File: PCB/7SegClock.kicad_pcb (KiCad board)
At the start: 2 copper layers, 177.8 x 76.2 mm, 144 parts, among them CON1 USB_Micro_Vertical, Q1 NPN, Q10 DMN2041LSD-13, Q11 DMN2041LSD-13, Q12 DMN2041LSD-13, Q13 DMN2041LSD-13, Q14 DMN2041LSD-13, Q15 DMN2041LSD-13, Q16 DMN2041LSD-13, Q17 DMN2041LSD-13, Q18 DMN2041LSD-13, Q19 DMN2041LSD-13, Q2 DMN2041LSD-13, Q20 DMN2041LSD-13, Q21 DMN2041LSD-13, Q22 DMN2041LSD-13, Q23 DMN2041LSD-13, Q24 DMN2041LSD-13, Q25 DMN2041LSD-13, Q26 DMN2041LSD-13, Q27 DMN2041LSD-13, Q28 DMN2041LSD-13, Q29 DMN2041LSD-13, Q3 DMN2041LSD-13, Q30 DMN2041LSD-13, Q31 DMN2041LSD-13, Q32 DMN2041LSD-13, Q4 DMN2041LSD-13, Q5 DMN2041LSD-13, Q6 DMN2041LSD-13, Q7 DMN2041LSD-13, Q8 DMN2041LSD-13, Q9 DMN2041LSD-13, U1 TPS62172DSGT, U2 P8X32A, U3 FT232RL, U4 24LC256, U5 DS3231, U6 LCMX02-640UHC-4TG144C, U7 Electric_Imp, X1 5mhz CRYSTAL

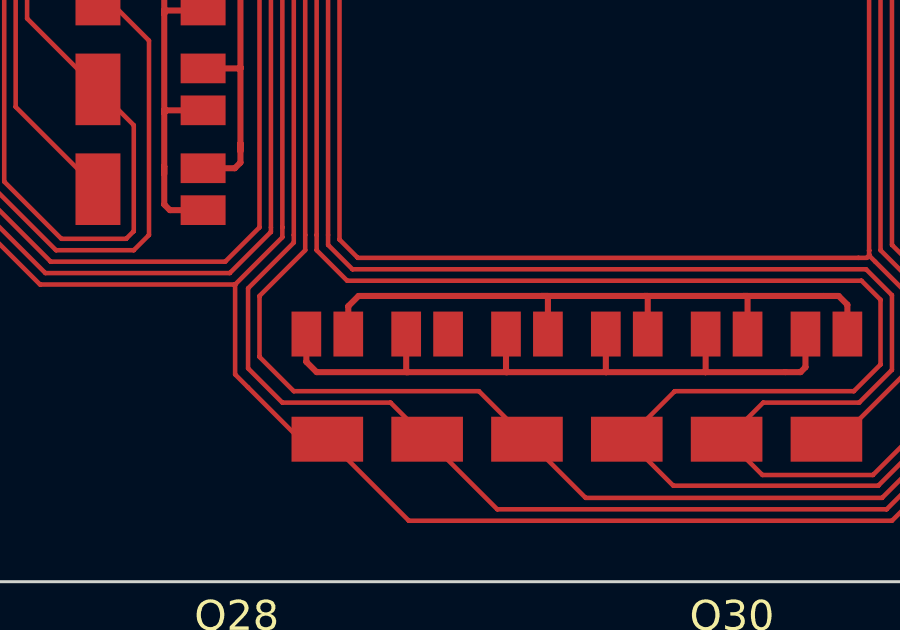
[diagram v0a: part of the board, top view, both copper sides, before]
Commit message: PCB work.
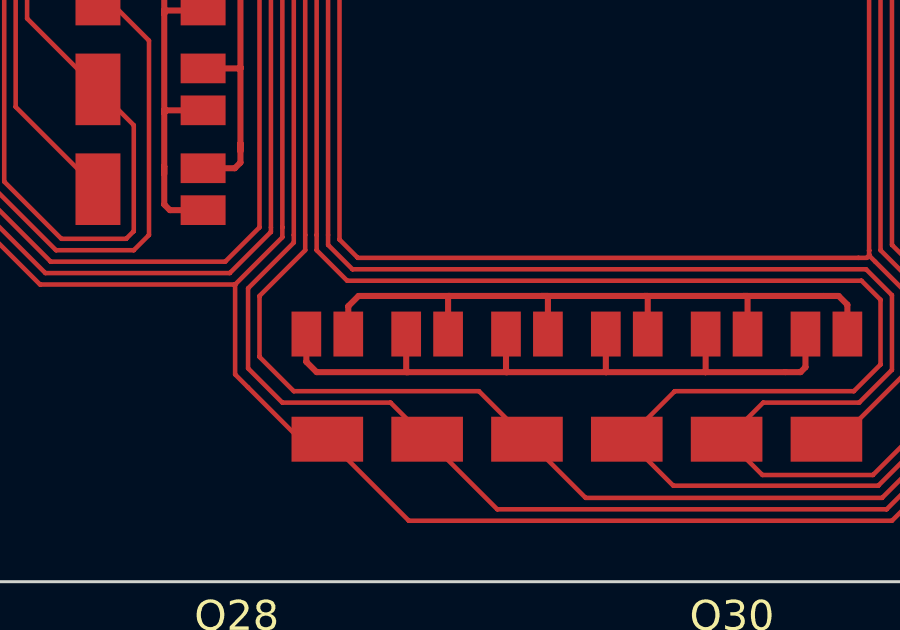
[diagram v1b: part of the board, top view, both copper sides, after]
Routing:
- net Net-(D3-Pad56): track 23.1 -> 24.4 mm
